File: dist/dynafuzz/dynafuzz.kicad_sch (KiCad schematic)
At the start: 54 parts, among them J1 AudioJack_IN, J2 AudioJack_OUT, J3 Jack-DC, Q1 Q_NPN, Q2 Q_NPN, Q3 Q_NPN, Q4 Q_NPN, SW1 SW_3PDT_x3

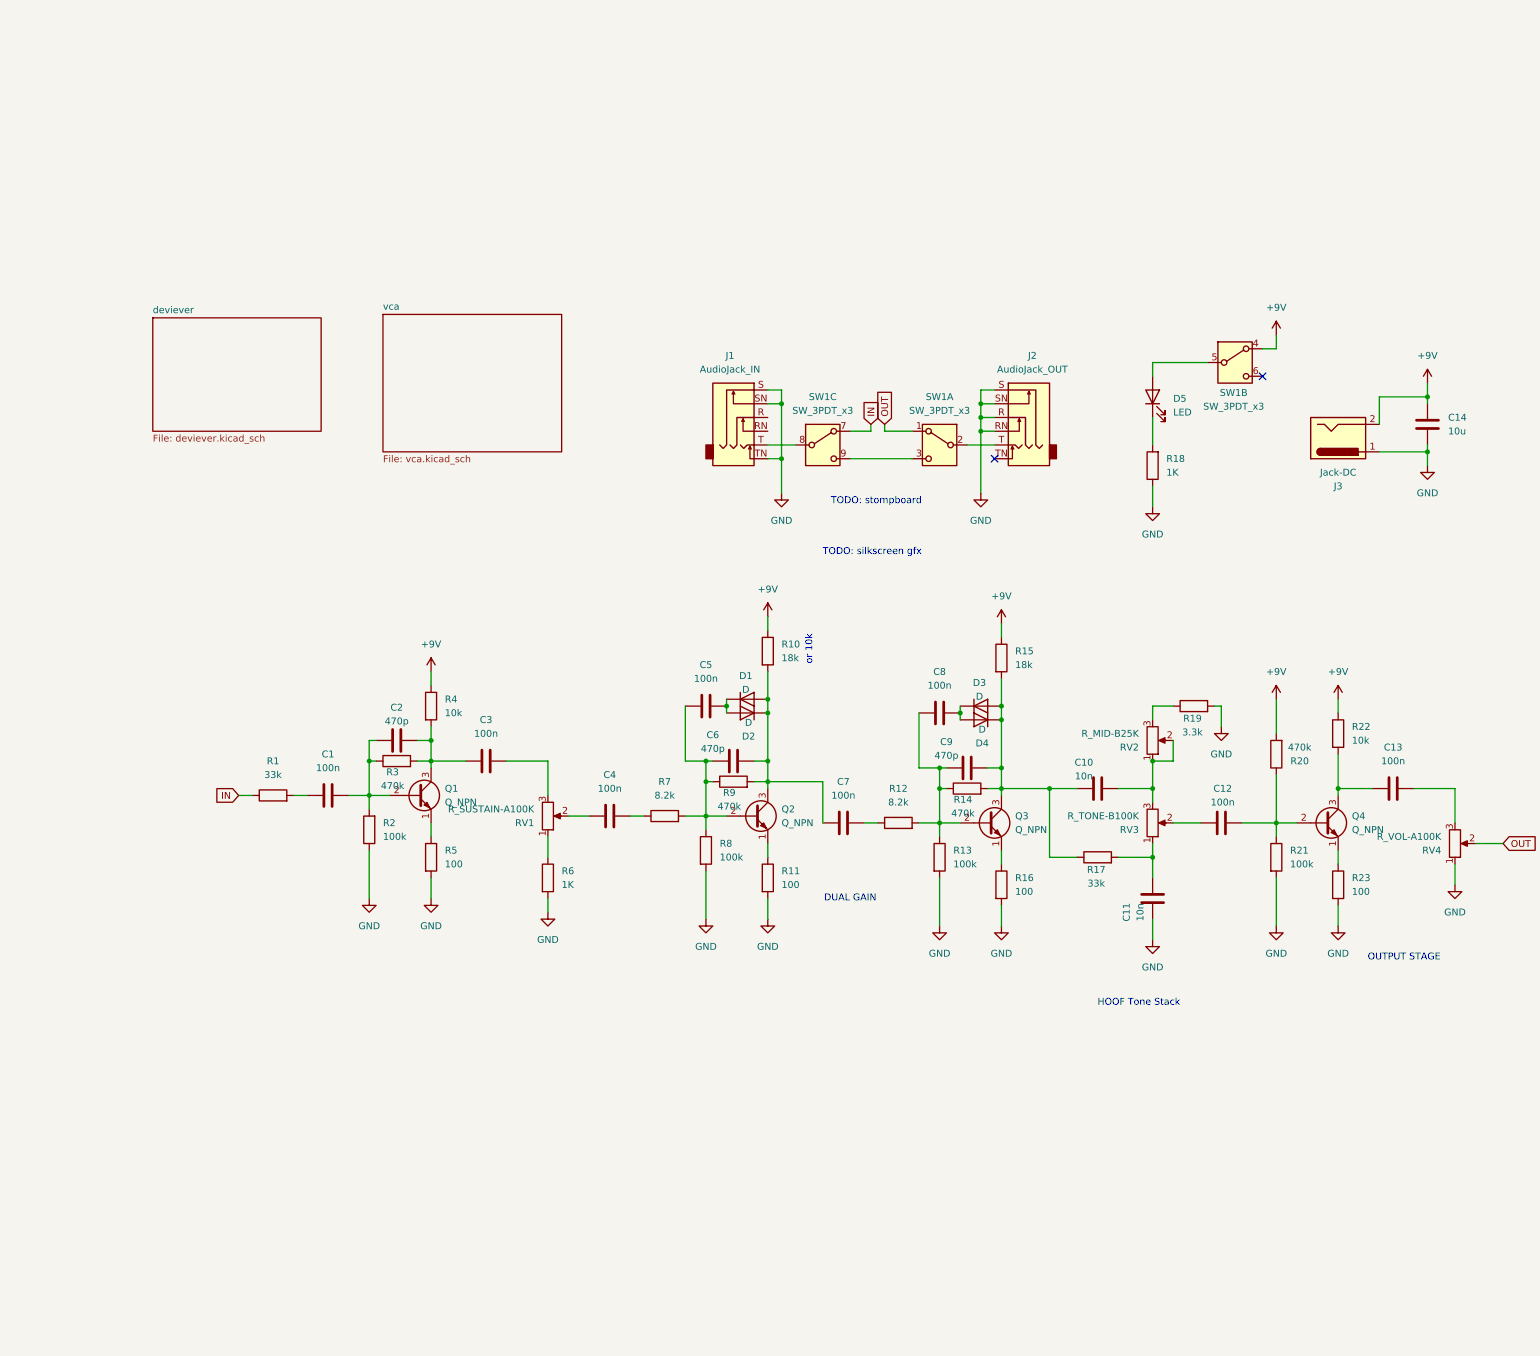
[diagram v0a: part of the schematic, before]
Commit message: board interconnect
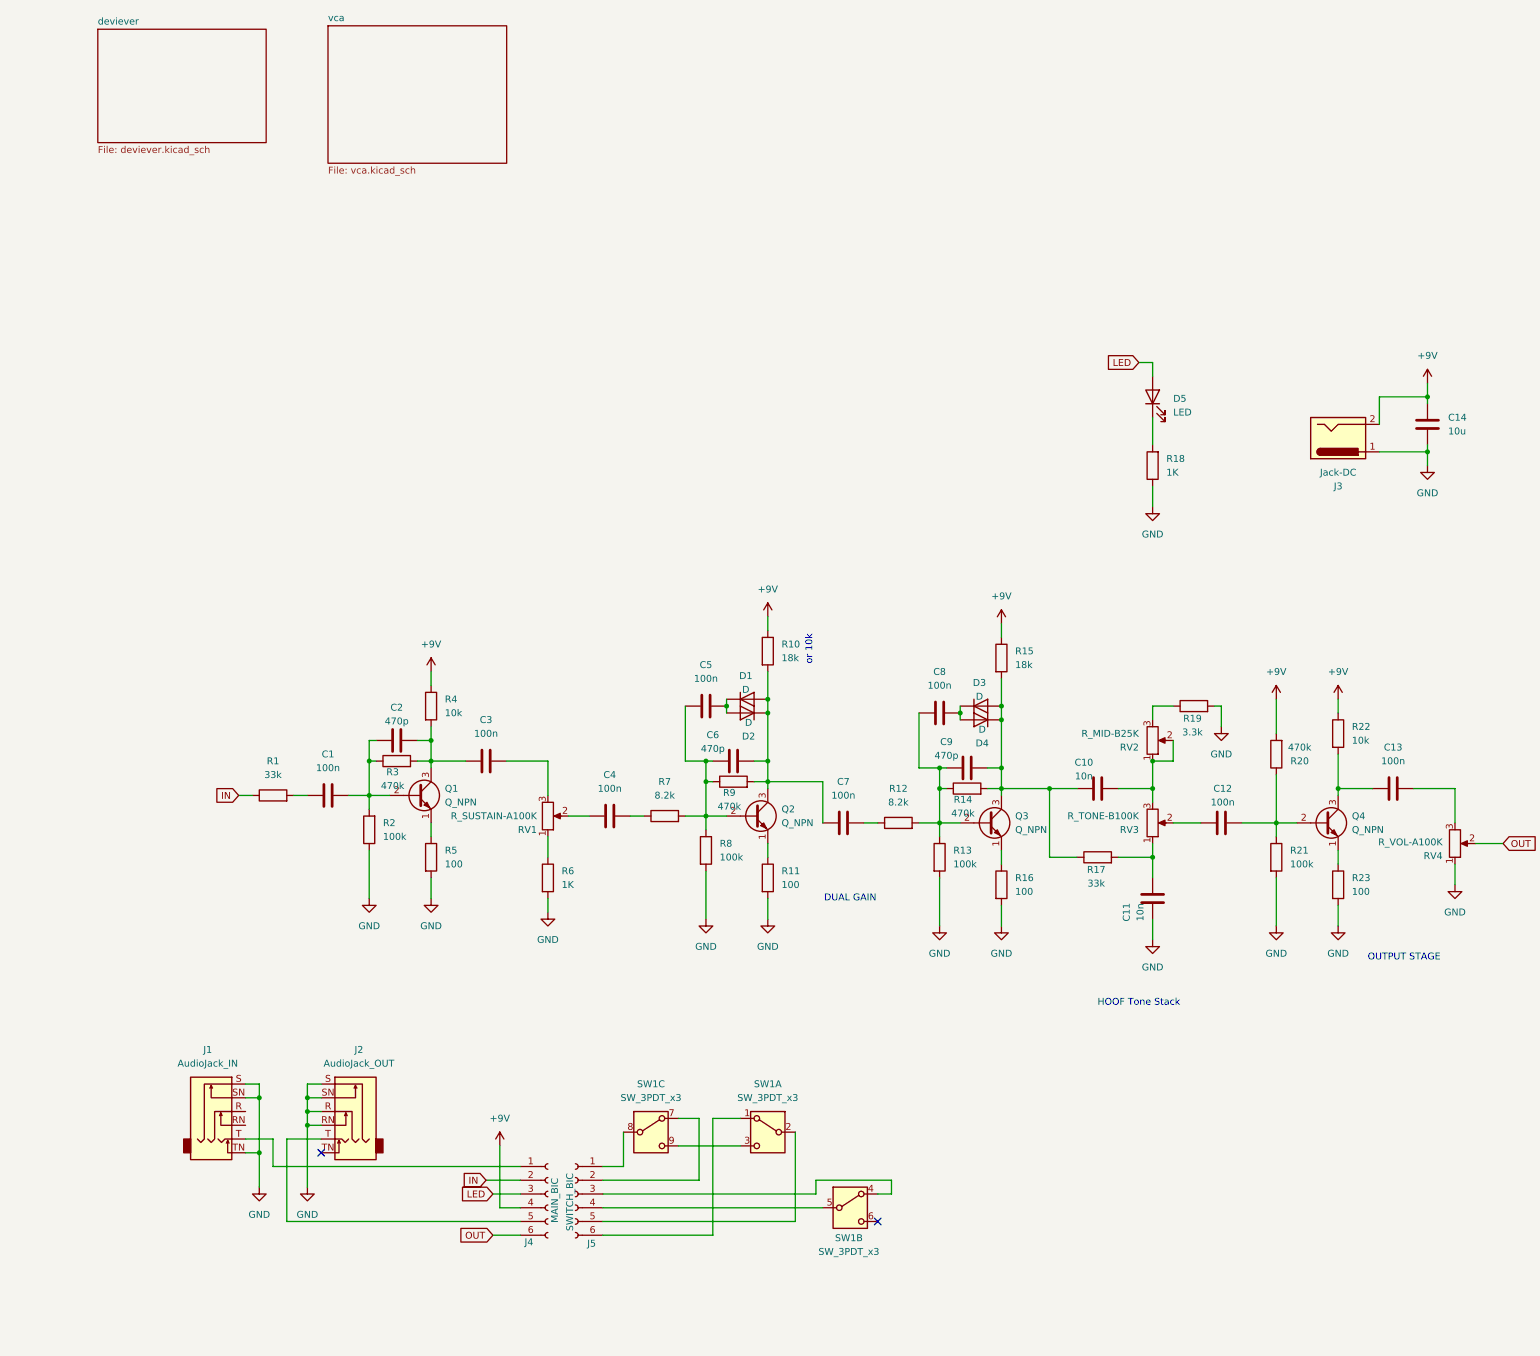
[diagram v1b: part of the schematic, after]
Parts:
- added J4: MAIN_BIC, Connector_PinSocket_2.54mm:PinSocket_1x06_P2.54mm_Vertical, symbol Connector:Conn_01x06_Socket
- added J5: SWITCH_BIC, Connector_PinSocket_2.54mm:PinSocket_1x06_P2.54mm_Vertical, symbol Connector:Conn_01x06_Socket
- SW1: footprint Connector_PinSocket_2.54mm:PinSocket_1x09_P2.54mm_Vertical -> _effects_shared_footprints:Stompbox Switch
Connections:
- net +9V: now also J4.4 (Pin_4); no longer SW1.4 (A)
- net IN: now also J4.2 (Pin_2); no longer SW1.7 (A)
- net OUT: now also J4.6 (Pin_6); no longer SW1.1 (A)
- net at SW1.5 (B): now also J5.4 (Pin_4); no longer D5.2 (A)
- net at SW1.8 (B): now also J5.1 (Pin_1); no longer J1.T
- net at SW1.2 (B): now also J5.5 (Pin_5); no longer J2.T
- new net: J5.2 (Pin_2), SW1.7 (A)
- new net: J5.6 (Pin_6), SW1.1 (A)
- new net: J2.T, J4.5 (Pin_5)
- new net: J5.3 (Pin_3), SW1.4 (A)
- new net: J1.T, J4.1 (Pin_1)
- new net LED: D5.2 (A), J4.3 (Pin_3)
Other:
- note removed: "TODO: silkscreen gfx"
- note removed: "TODO: stompboard"
- moved on the sheet: J1, J2, SW1A, SW1B, SW1C
